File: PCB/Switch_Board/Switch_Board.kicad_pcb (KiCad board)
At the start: 2 copper layers, 99.8 x 99.8 mm, 9 parts

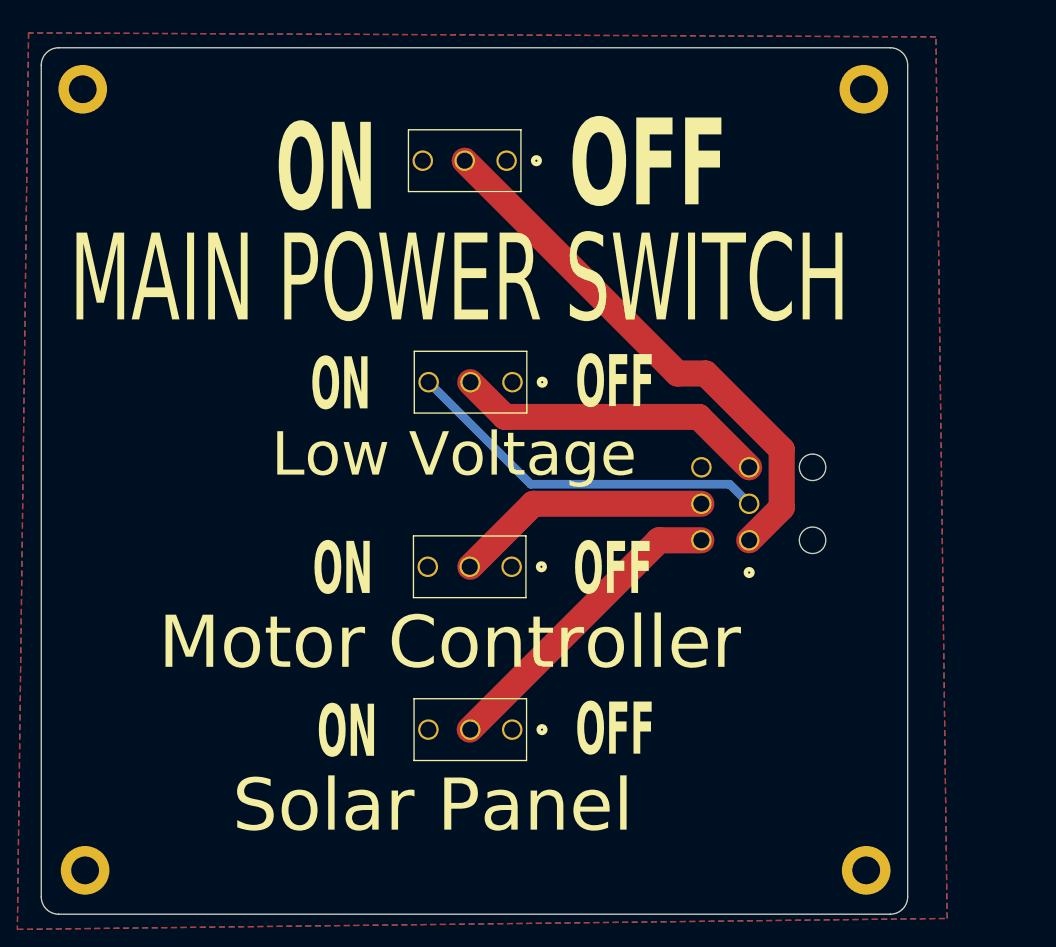
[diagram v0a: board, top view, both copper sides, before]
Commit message: Updated_Final_0418
Not including image yet, but it is the final board
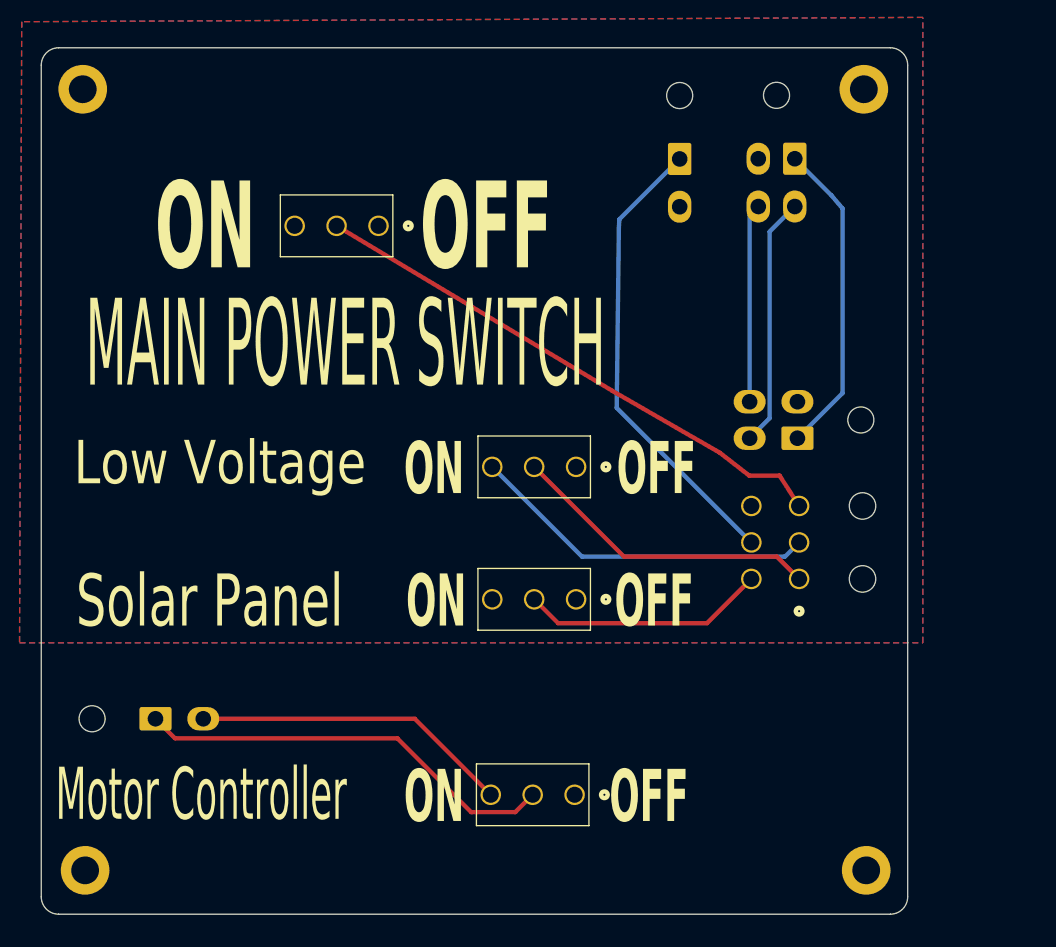
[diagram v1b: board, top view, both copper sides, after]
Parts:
- added ESTOP1: Conn_01x02, Connector_Molex:Molex_Mini-Fit_Jr_5569-02A2_2x01_P4.20mm_Horizontal, B.Cu at (140.8, 50.3)
- added J1: Conn_01x04_Pin, Connector_Molex:Molex_Mini-Fit_Jr_5569-04A2_2x02_P4.20mm_Horizontal, B.Cu at (154.3, 82.5)
- added J4: Conn_01x04_Pin, Connector_Molex:Molex_Mini-Fit_Jr_5569-04A2_2x02_P4.20mm_Horizontal, B.Cu at (154.0, 50.3)
- added MotorControllerEN1: Conn_01x02, Connector_Molex:Molex_Mini-Fit_Jr_5569-02A2_2x01_P4.20mm_Horizontal, B.Cu at (80.4, 114.8)
- HV1: renamed from Main Power Switch
- moved MotorController1 27.2 mm to (128.7, 123.5)
- moved SolarPanel1 16.7 mm to (128.8, 101.0)
- moved HV1 16.5 mm to (106.1, 58.0)
- moved LV1 12.2 mm to (128.8, 85.8)
- moved Switch1 7.27 mm to (154.5, 98.6)
- renumbered LowVoltage to LV1, MotorController to MotorController1, SolarPanel to SolarPanel1
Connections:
- net Net-(LV1-A) renamed /LV_EN_SIGNAL
- net Net-(SolarPanel1-B) renamed /Solar_EN
- HV1 pad 2: Net-(HV1-B) -> /HV_EN
- LV1 pad 2: Net-(LV1-B) -> /LV_EN_PWR
- MotorController1 pad 3: GND -> Net-(MotorController1-A)
- Switch1 pad 1: Net-(HV1-B) -> /LV_EN_PWR
- Switch1 pad 3: Net-(LV1-B) -> /HV_EN
- Switch1 pad 5: Net-(MotorController1-B) -> /ESTOP
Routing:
- net /HV_EN: track 0.00 -> 63.2 mm
- net Net-(HV1-B): track 62.3 -> 0.00 mm
- net /ESTOP: track 0.00 -> 53.5 mm
- net Net-(MotorController1-A): track 0.00 -> 36.7 mm
- net +12V: track 0.00 -> 36.5 mm
- net Net-(LV1-B): track 36.2 -> 0.00 mm
- net /LV_EN_PWR: track 0.00 -> 35.8 mm
- net /CANH1: track 0.00 -> 28.8 mm
- net /CANL1: track 0.00 -> 22.9 mm
- net Net-(MotorController1-B): track 29.6 -> 48.7 mm
- net /Solar_EN: track 35.7 -> 28.3 mm
- net /LV_EN_SIGNAL: track 42.7 -> 40.3 mm
- net unconnected-(LV1-C-Pad1): track 0.71 -> 0.00 mm
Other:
- board text added: "(symbol "LOGO" (pin_names (offset 1.016)) (in_bom yes) (on_board yes) (property "Reference" "#G" (at 0 396.24 0) (effects (font (size 1.27 1.27)) hide) ) (property "Value" "LOGO" (at 0 -396.24 0) (effects (font (size 1.27 1.27)) hide) ) (property "Footprint" "" (at 0 0 0) (effects (font (size 1.27 1.27)) hide) ) (property "Datasheet" "" (at 0 0 0) (effects (font (size 1.27 1.27)) hide) ) (symbol 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"
- board text added: "6_PIN SWITCH"
- board text added: "CAN1"
- board text added: "CAN2"
- board text added: "ESTOP"
- board text added: "LOW VOLTAGE"
- board text added: "MAIN POWER"
- board text added: "MOTOR CONTROLLER"
- board text added: "Motor_Controller"
- board text added: "Noora Kumar | BSEE '29 | www.linkedin.com/in/noorakumar/"
- board text added: "SOLAR PANEL"

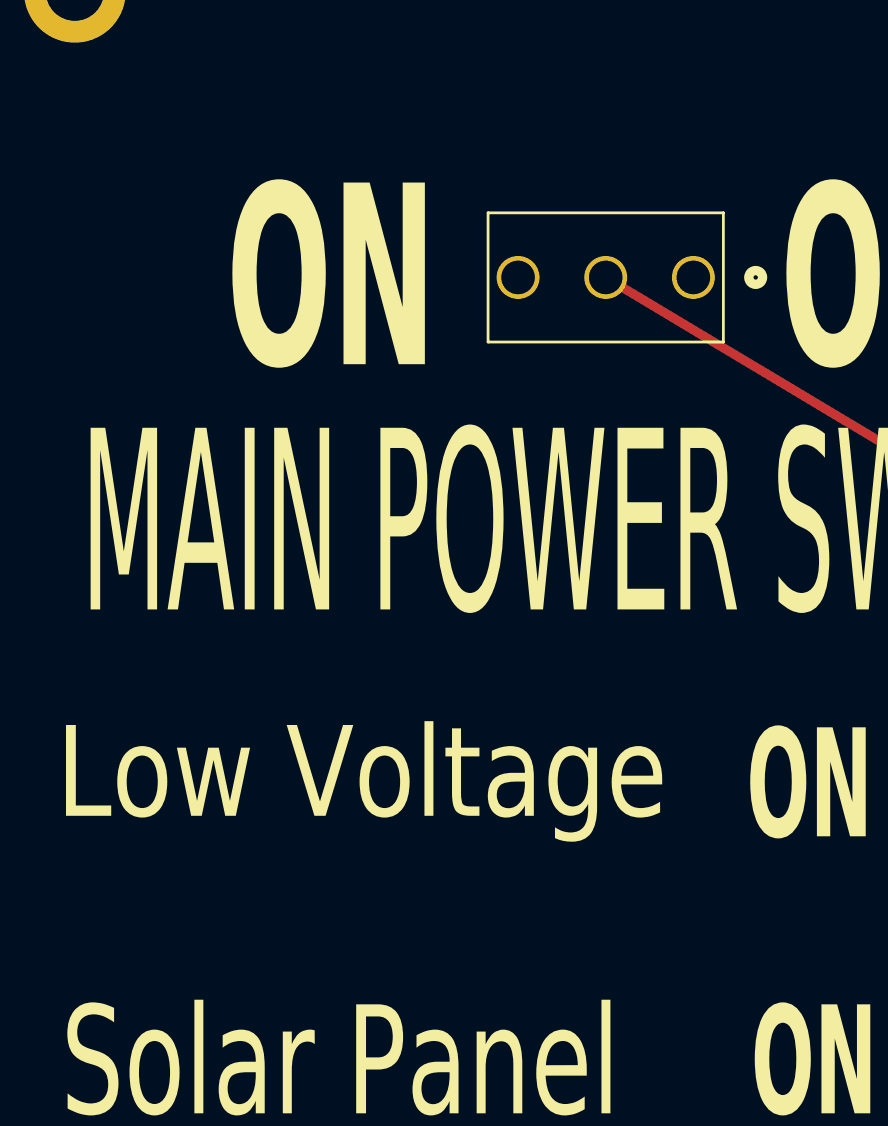
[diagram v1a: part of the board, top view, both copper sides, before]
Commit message: SpritesAdded_0418
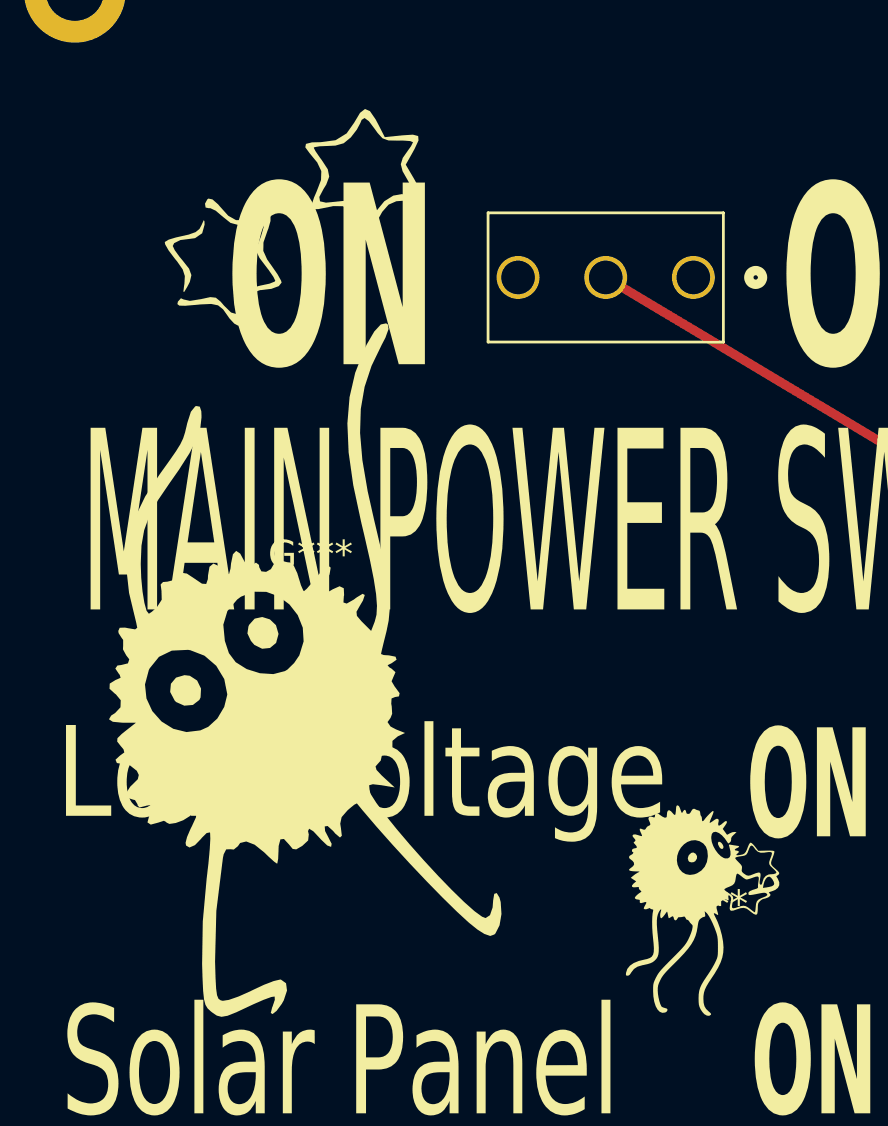
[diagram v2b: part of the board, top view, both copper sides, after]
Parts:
- added G***: LOGO, LOGO, F.Cu at (85.0, 73.2)
- added G***: LOGO, LOGO, F.Cu at (106.8, 92.5)
